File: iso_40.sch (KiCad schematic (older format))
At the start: 14 parts

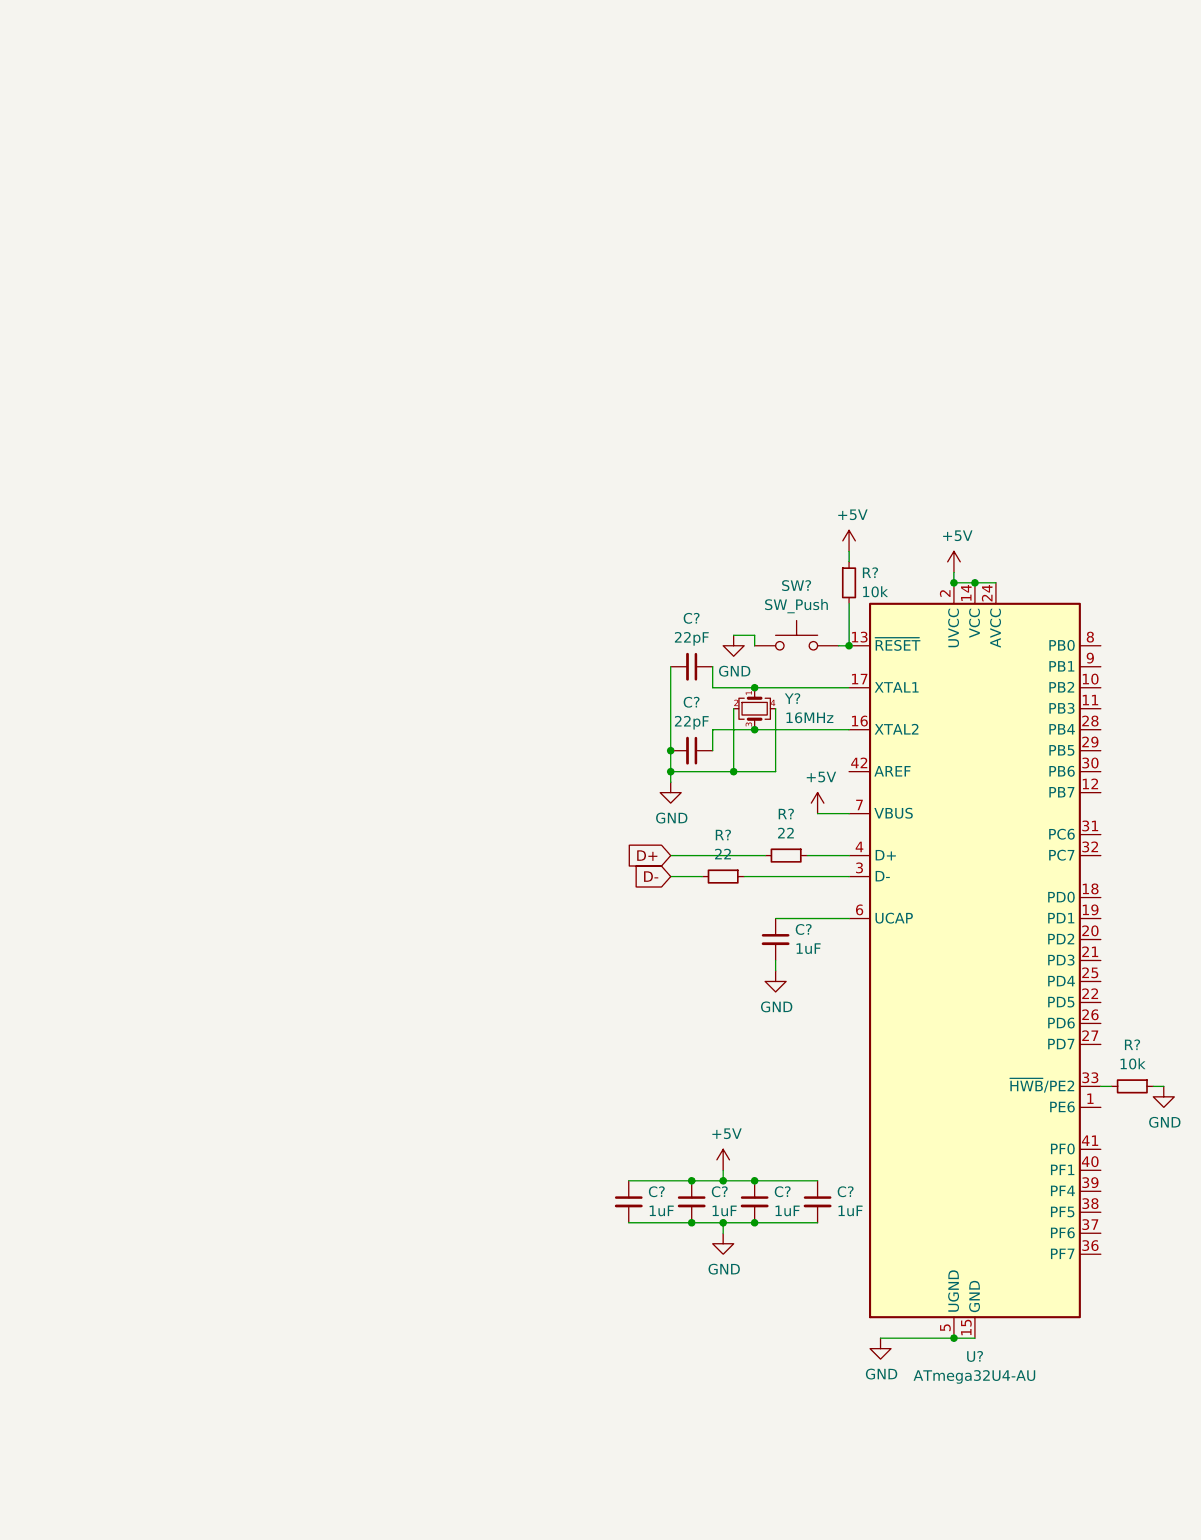
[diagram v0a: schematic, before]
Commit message: layout png
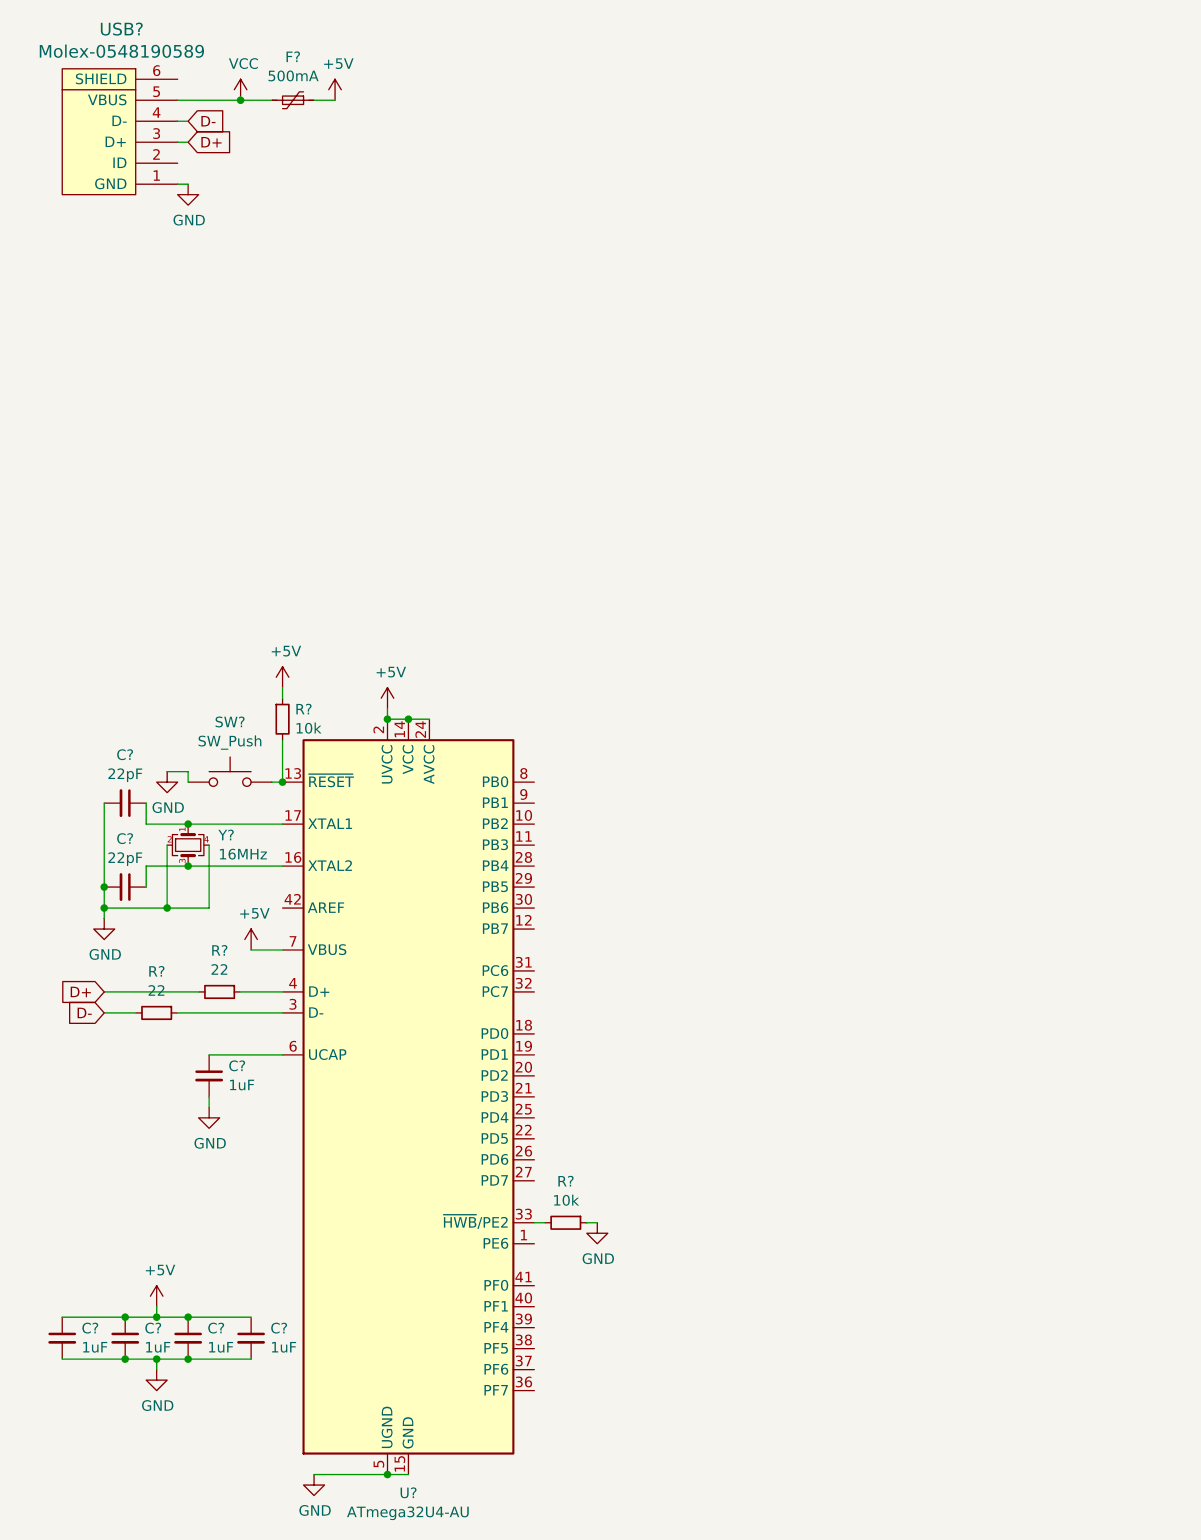
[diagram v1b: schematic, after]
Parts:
- added F?: 500mA, symbol Device:Polyfuse_Small
- added USB?: Molex-0548190589, symbol random-keyboard-parts:Molex-0548190589
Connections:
- net +5V: now also F?.1
- net D+: now also USB?.3 (D+)
- net D-: now also USB?.4 (D-)
- net GND: now also USB?.1 (GND)
- new net VCC: F?.2, USB?.5 (VBUS)
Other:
- moved on the sheet: C?, R?, SW?, U?, Y?
